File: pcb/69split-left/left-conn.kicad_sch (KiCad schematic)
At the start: 1 part, among them J3 USB_C_Receptacle_USB2.0_16P

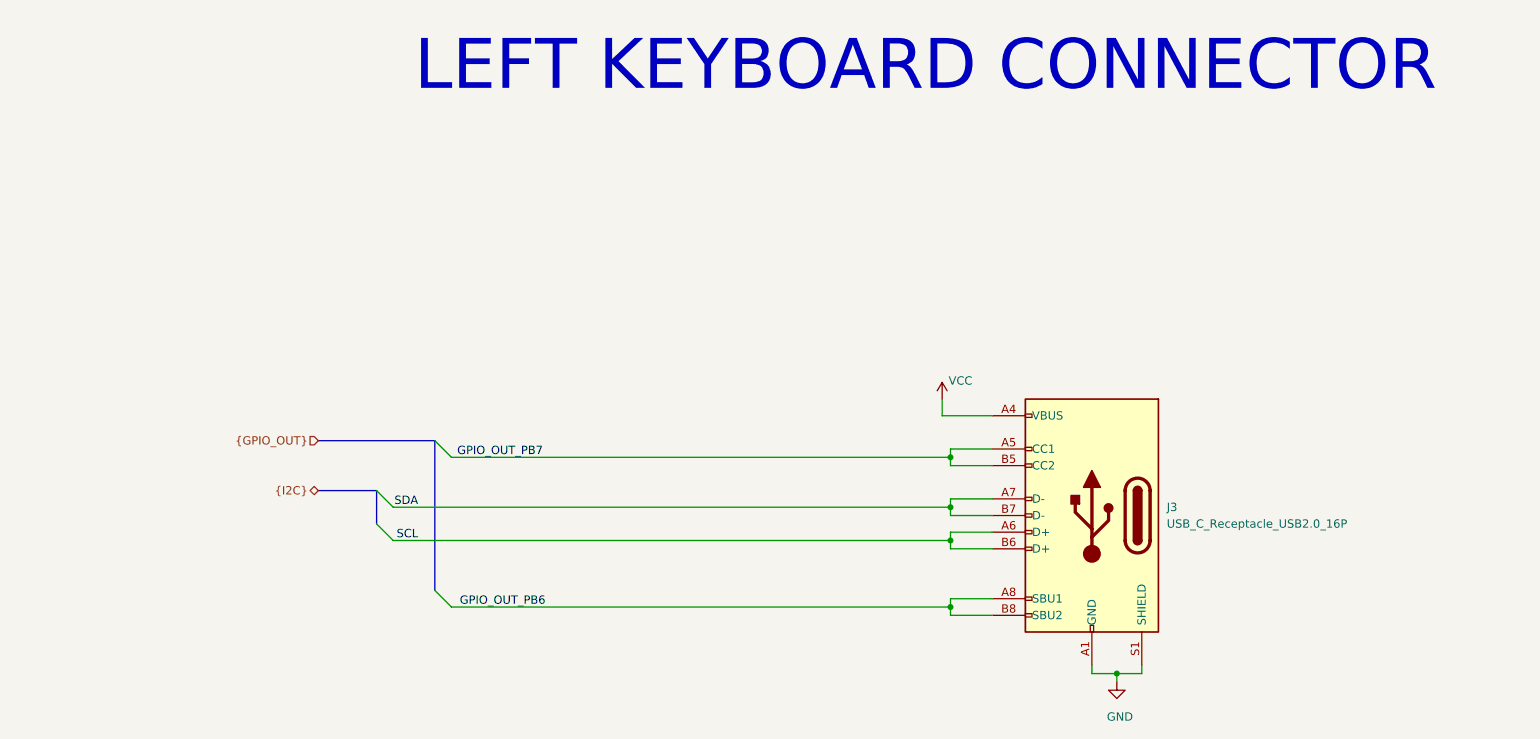
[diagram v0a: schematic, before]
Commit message: Final touches.
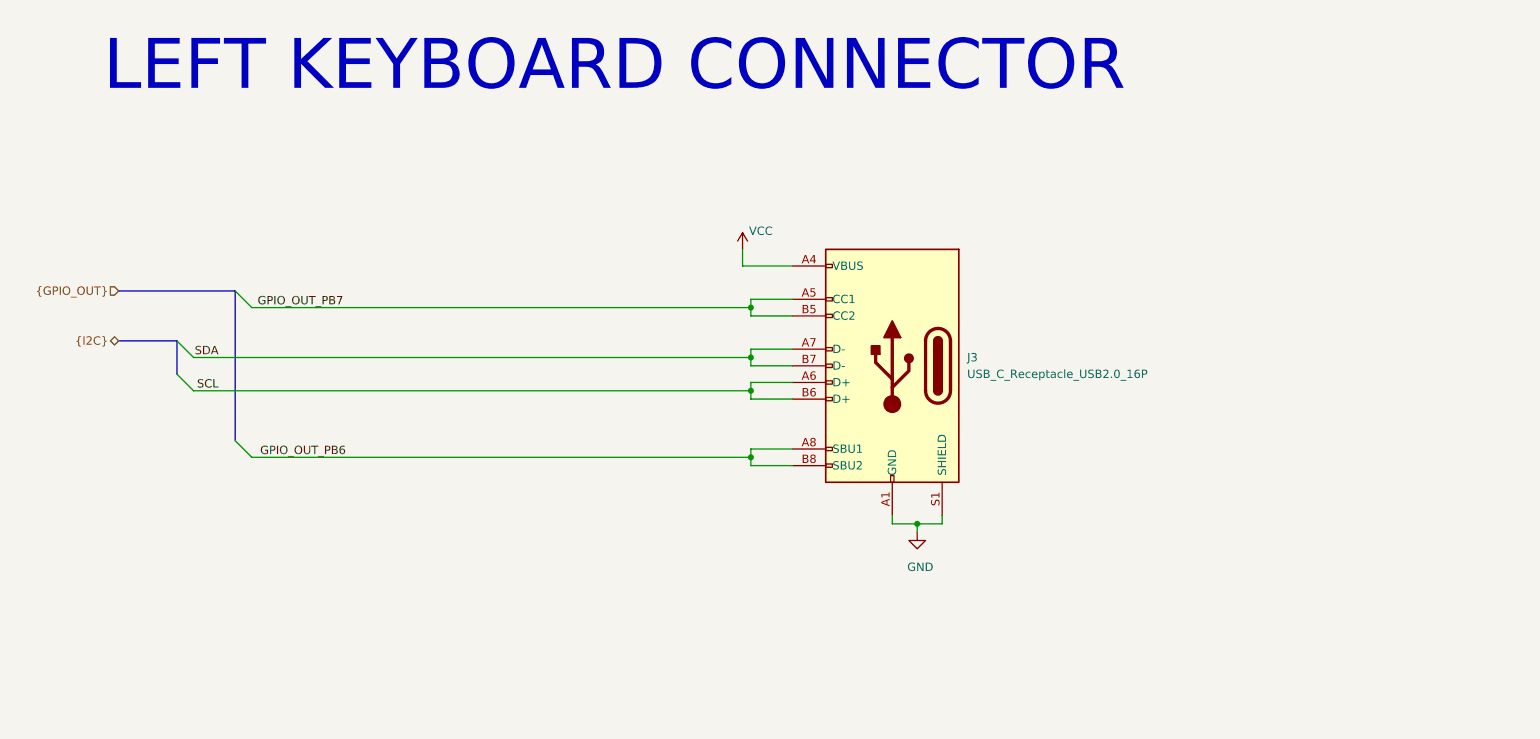
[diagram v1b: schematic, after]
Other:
- moved on the sheet: J3
